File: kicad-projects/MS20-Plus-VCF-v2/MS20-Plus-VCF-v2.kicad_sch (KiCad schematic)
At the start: 78 parts

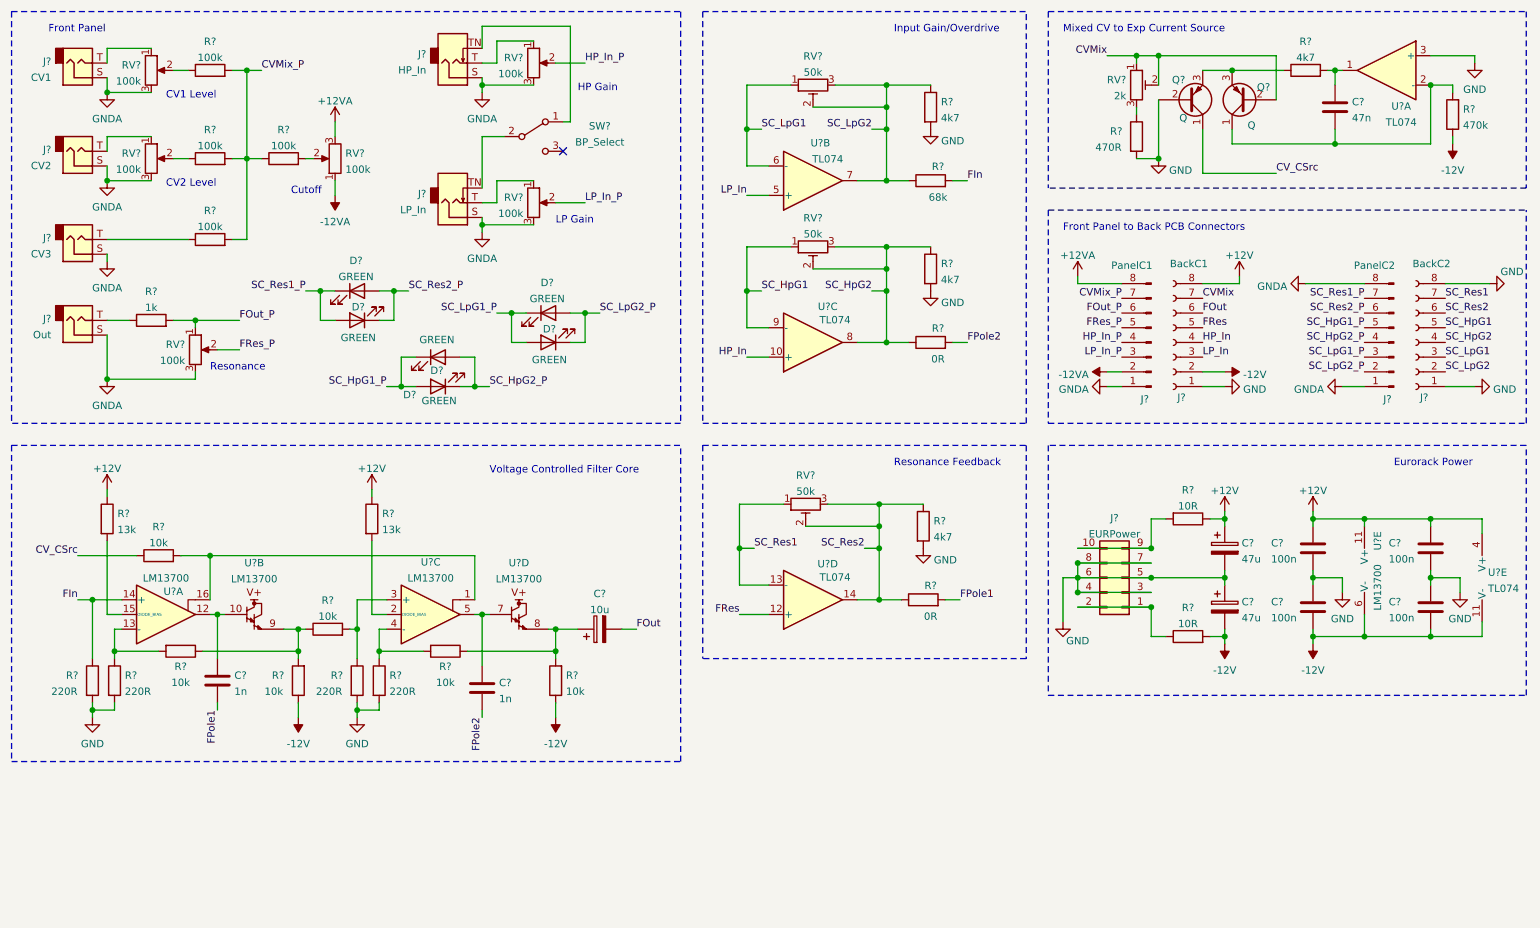
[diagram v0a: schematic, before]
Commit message: Minor cleanups
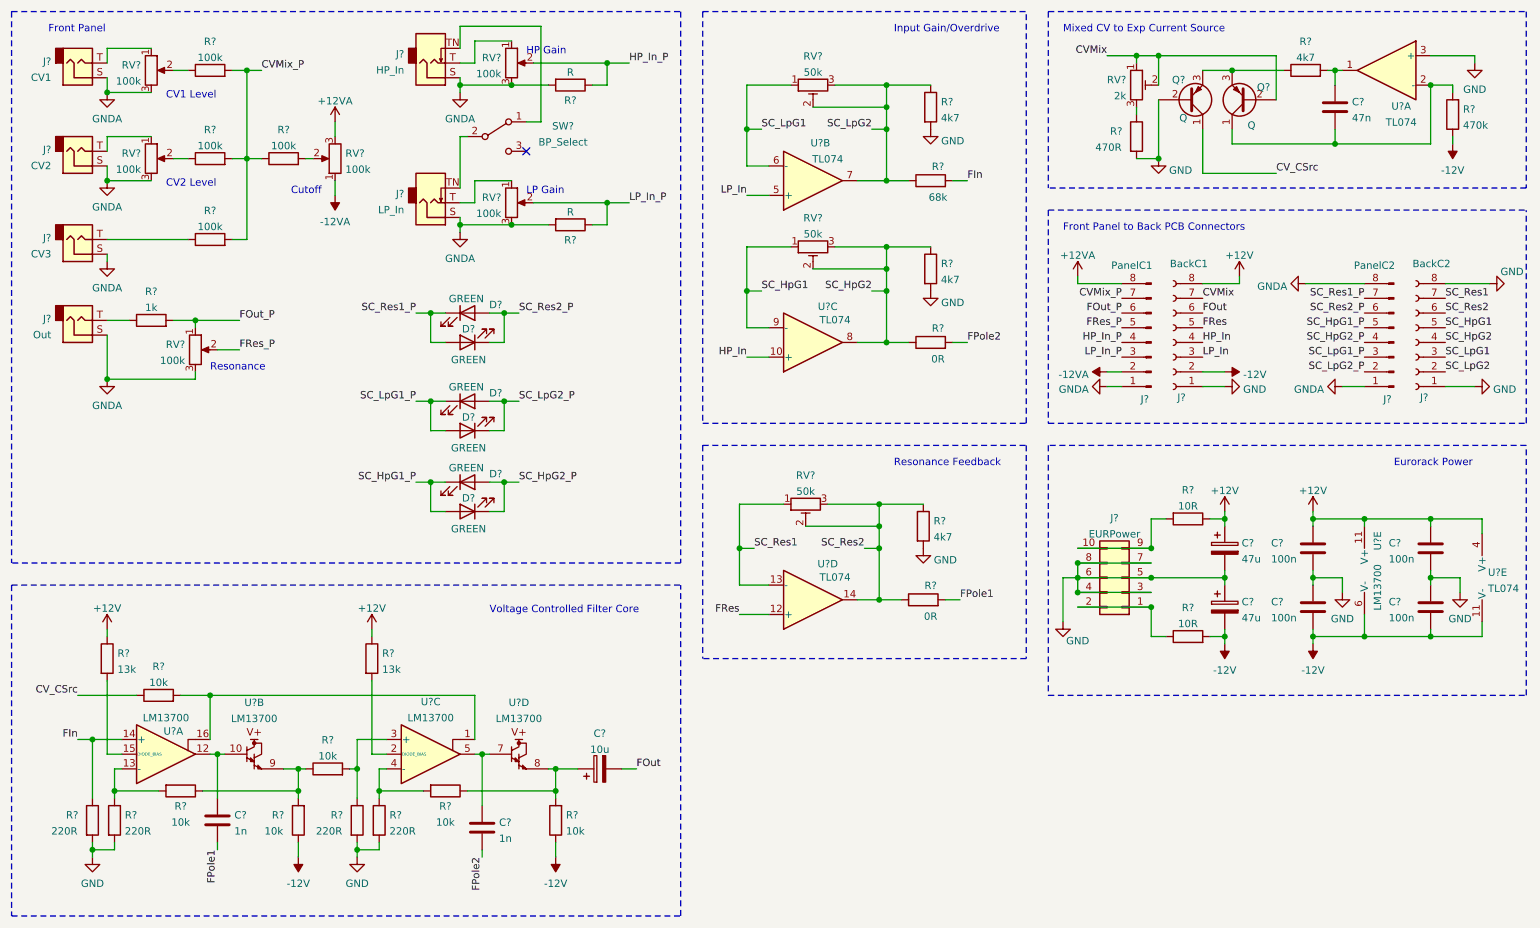
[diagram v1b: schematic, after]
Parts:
- added R? (x2): R, symbol Device:R
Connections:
- net GNDA: now also R?.2, R?.2
- net HP_In_P: now also R?.1
- net LP_In_P: now also R?.1
- net SC_HpG1_P: now also D?.1 (K), D?.2 (A); no longer D?.1 (K), D?.2 (A)
- net SC_HpG2_P: now also D?.1 (K), D?.2 (A); no longer D?.1 (K), D?.2 (A)
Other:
- moved on the sheet: C?, D?, J?, R?, RV?, SW?, U?A, U?B, U?C, U?D
